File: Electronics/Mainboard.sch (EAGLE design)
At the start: 37 parts, among them IC1 4081N, IC2 4069N, Q1 IRFZ48V, Q2 IRF4905V, Q3 IRFZ48V, Q4 IRF4905V, Q5 IRFZ48V, Q6 IRF4905V, Q7 IRFZ48V, Q8 IRF4905V, X3 24V Batt

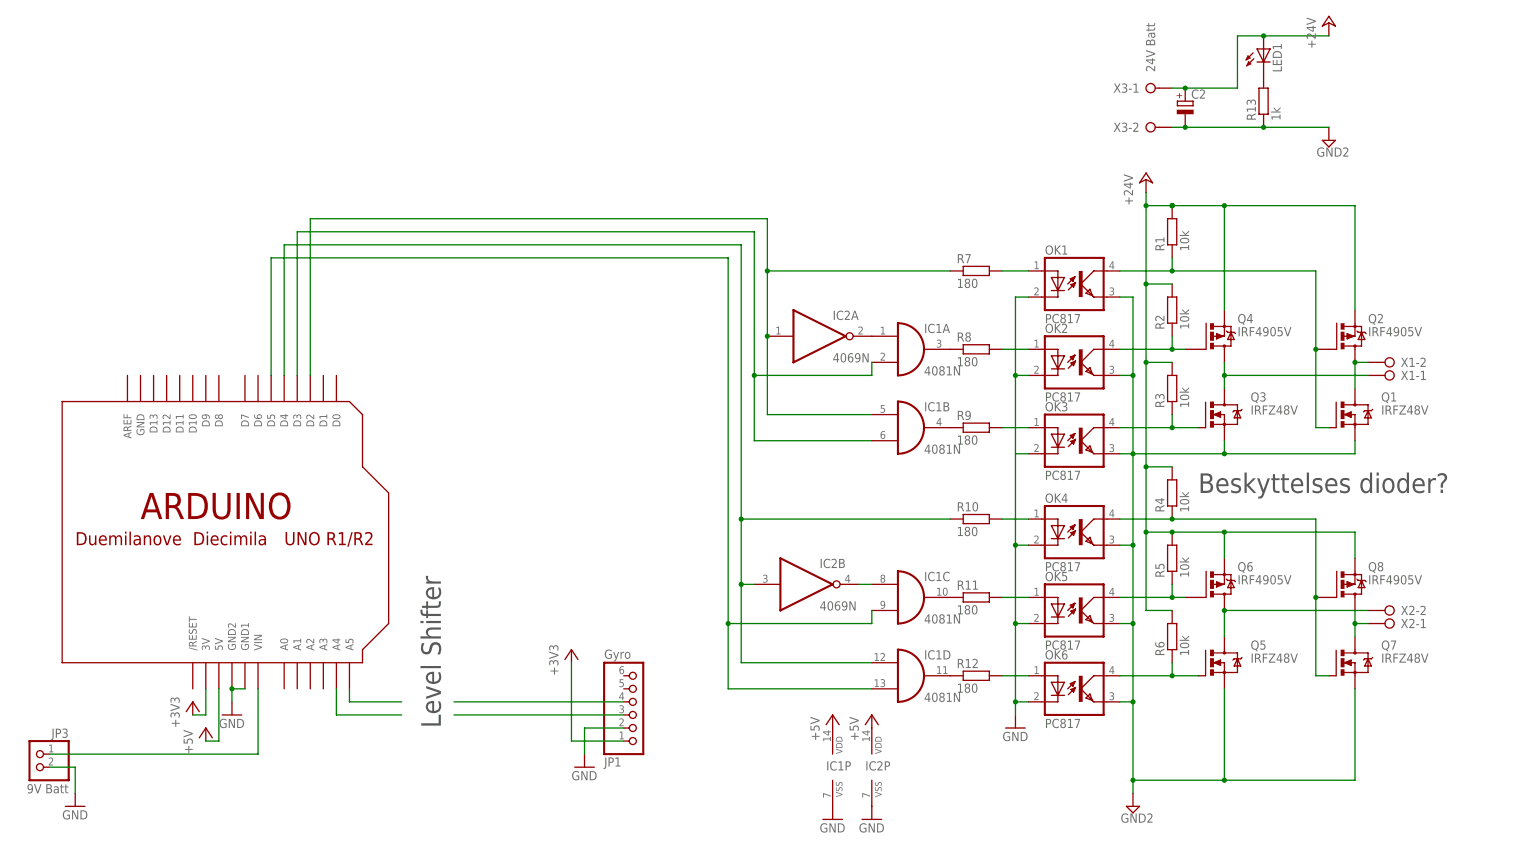
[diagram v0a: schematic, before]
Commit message: 
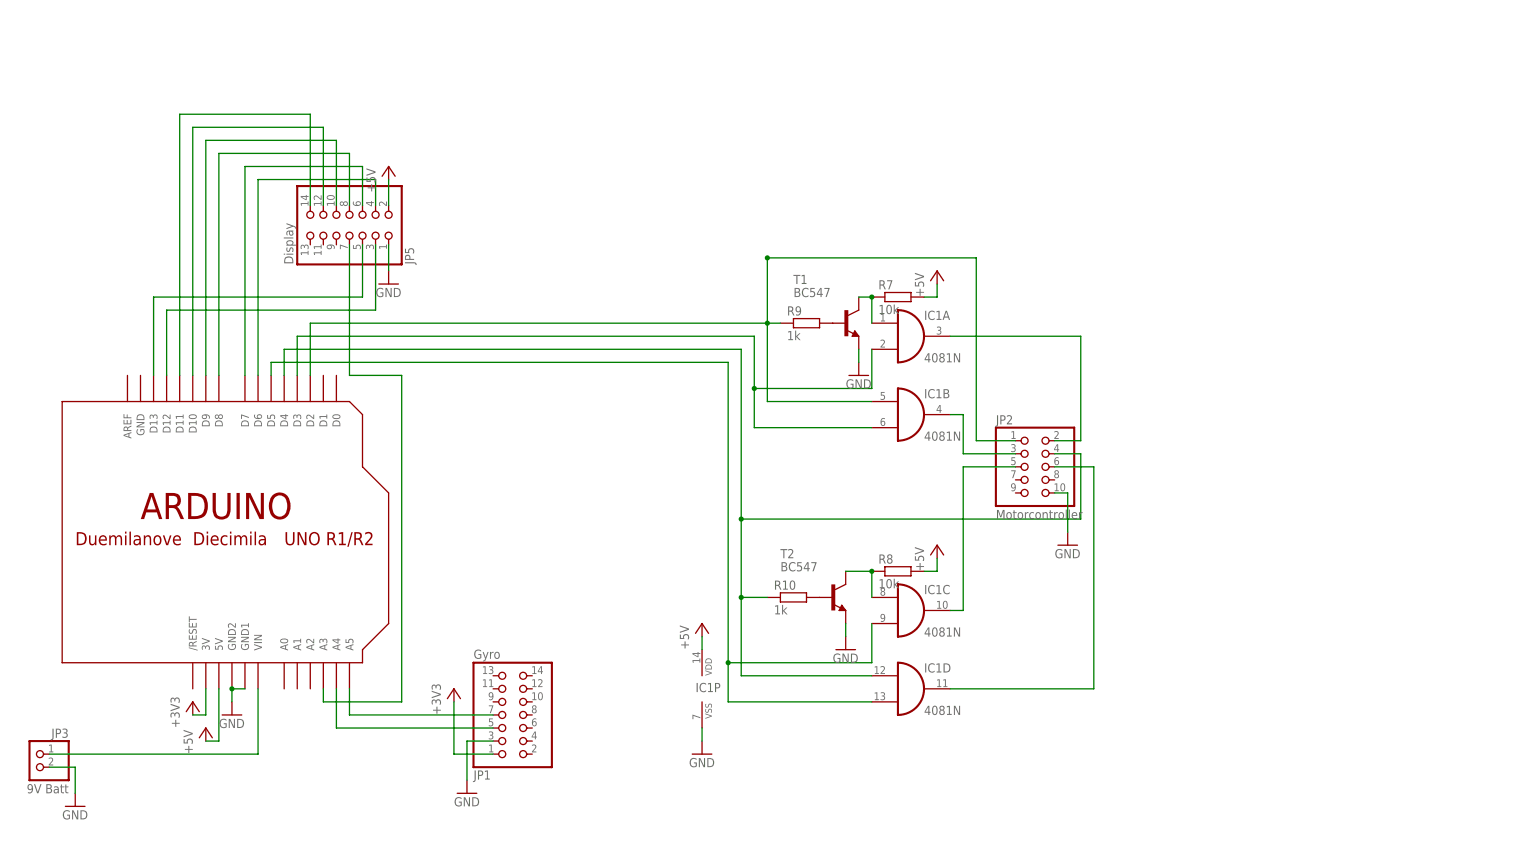
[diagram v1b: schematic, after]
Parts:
- removed C2: (no value), rcl:CPOL-EUE5-10.5
- removed IC2: 4069N, 40xx:4069N
- removed LED1: (no value), led:LED5MM
- removed OK1, OK2, OK3, OK4, OK5, OK6: PC817, optocoupler:PC817
- removed Q1, Q3, Q5, Q7: IRFZ48V, transistor-power:IRFZ48V
- removed Q2, Q4, Q6, Q8: IRF4905V, transistor-power:IRF4905V
- removed R1, R2, R3, R4, R5, R6: 10k, rcl:R-EU_0207/10
- removed R11, R12: 180, rcl:R-EU_0207/10
- removed R13: 1k, rcl:R-EU_0207/10
- removed X1, X2: (no value), con-wago-508:W237-02P
- removed X3: 24V Batt, con-wago-508:W237-02P
- added JP2: Motorcontroller, pinhead:PINHD-2X5
- added JP5: Display, pinhead:PINHD-2X7
- added T1, T2: BC547, transistor:BC547
- JP1: device pinhead:PINHD-1X6 -> pinhead:PINHD-2X7
- R10, R9: value 180 -> 1k
- R7, R8: value 180 -> 10k
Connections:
- removed net +24V: C2.+, LED1.A, Q2.S, Q4.S, Q6.S, Q8.S, R1.2, R2.2, R3.2, R4.2, R5.2, R6.2, X3-1.KL
- removed net GND2: C2.-, OK1.EMIT, OK2.EMIT, OK3.EMIT, OK4.EMIT, OK5.EMIT, OK6.EMIT, Q1.S, Q3.S, Q5.S, Q7.S, R13.1, X3-2.KL
- removed net N$12: OK1.COL, Q1.G, Q2.G, R1.1
- removed net N$13: OK3.COL, Q3.G, R3.1
- removed net N$14: OK3.A, R9.2
- removed net N$15: IC1A.O, R8.1
- removed net N$18: Q7.D, Q8.D, X2-1.KL
- removed net N$19: OK4.COL, Q7.G, Q8.G, R4.1
- removed net N$21: OK5.COL, Q6.G, R5.1
- removed net N$22: OK6.COL, Q5.G, R6.1
- removed net N$23: OK6.A, R12.2
- removed net N$24: IC1C.O, R11.1
- removed net N$25: IC1D.O, R12.1
- removed net N$27: IC1D.I0, IC2B.I, R10.1, U$1.D4
- removed net N$28: OK1.A, R7.2
- removed net N$6: LED1.C, R13.2
- removed net N$9: OK2.COL, Q4.G, R2.1
- removed net VCC: IC1P.VDD, IC2P.VDD, U$1.5V
- new net +5V: IC1P.VDD, JP5.2, R7.2, R8.2, U$1.5V
- new net N$31: JP5.4, U$1.D6
- new net N$38: JP5.8, U$1.D8
- new net N$40: JP5.10, U$1.D9
- new net N$43: JP5.14, U$1.D11
- new net N$44: JP5.3, U$1.D12
- new net N$45: JP5.5, U$1.D13
- new net N$46: JP5.7, U$1.A3
- net GND: now also JP1.3, JP2.10, JP5.1, T1.E, T2.E; no longer IC2P.VSS, JP1.2, OK1.C, OK2.C, OK3.C, OK4.C, OK5.C, OK6.C
- net N$1: now also IC1A.O, JP2.2; no longer Q5.D, Q6.D, X2-2.KL
- net N$10: now also JP2.1, R9.1; no longer IC2A.I, R7.1
- net N$16: now also R8.1, T2.C; no longer IC2B.O
- net N$17: now also R9.2, T1.B; no longer IC1B.O, R9.1
- net N$2: now also IC1B.O, JP2.3; no longer Q3.D, Q4.D, X1-1.KL
- net N$20: now also R10.2, T2.B; no longer OK5.A, R11.2
- net N$26: now also JP1.7
- net N$3: now also IC1D.I0, JP2.4, R10.1, U$1.D4; no longer OK2.A, R8.2
- net N$37: now also JP5.6, U$1.D7; no longer U$1.A4
- net N$4: now also IC1C.O, JP2.5; no longer Q1.D, Q2.D, X1-2.KL
- net N$41: now also JP1.5, U$1.A4; no longer JP1.3
- net N$42: now also JP5.12, U$1.D10; no longer JP1.4
- net N$5: now also IC1D.O, JP2.6; no longer OK4.A, R10.2
- net N$8: now also R7.1, T1.C; no longer IC2A.O
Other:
- note removed: "Beskyttelses dioder?"
- note removed: "Level Shifter"
- moved on the sheet: IC1A, IC1B, IC1C, IC1D, IC1P, R10, R7, R8, R9
